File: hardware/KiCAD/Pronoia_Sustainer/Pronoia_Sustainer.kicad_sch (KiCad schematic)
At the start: 0 parts

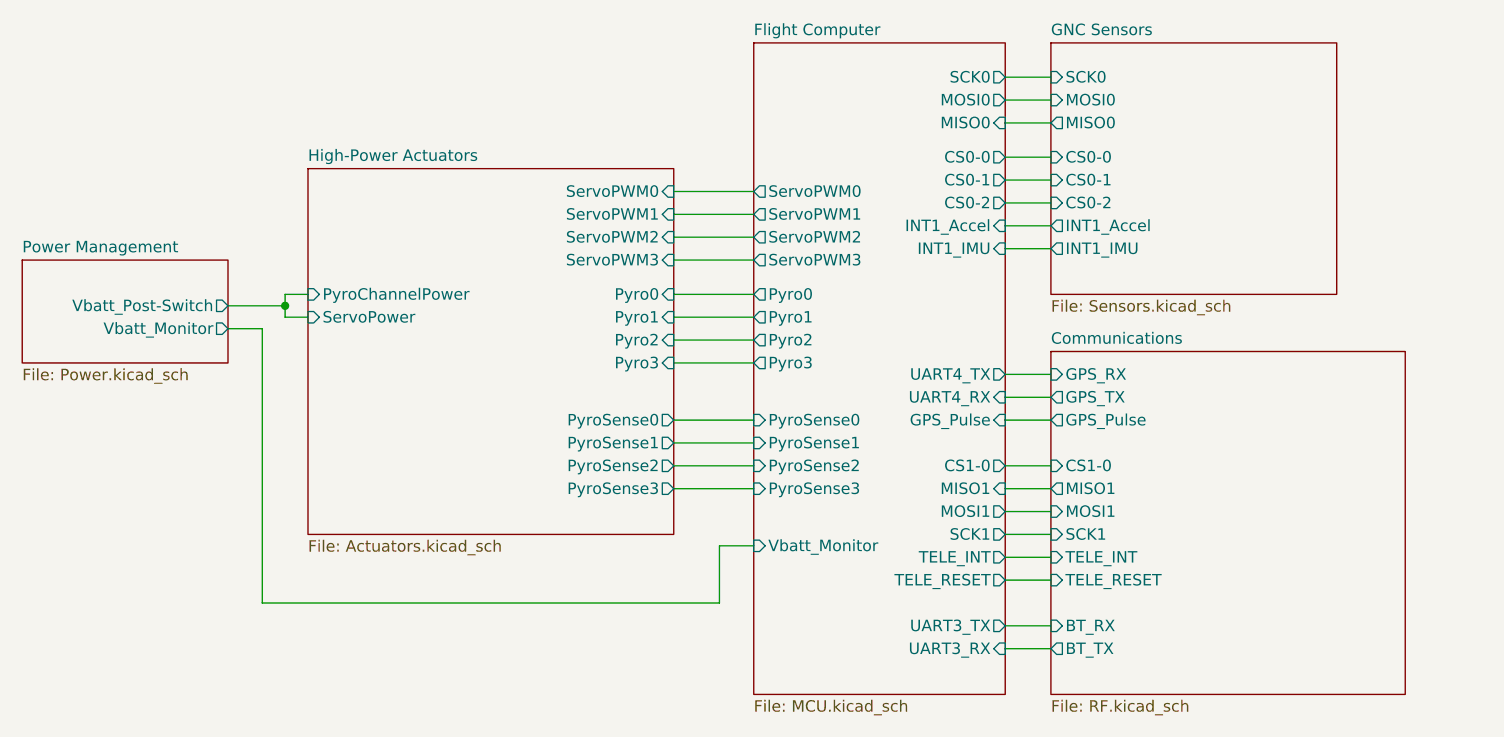
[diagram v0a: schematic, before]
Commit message: Finalized v2.0 of Pronoia Schematic
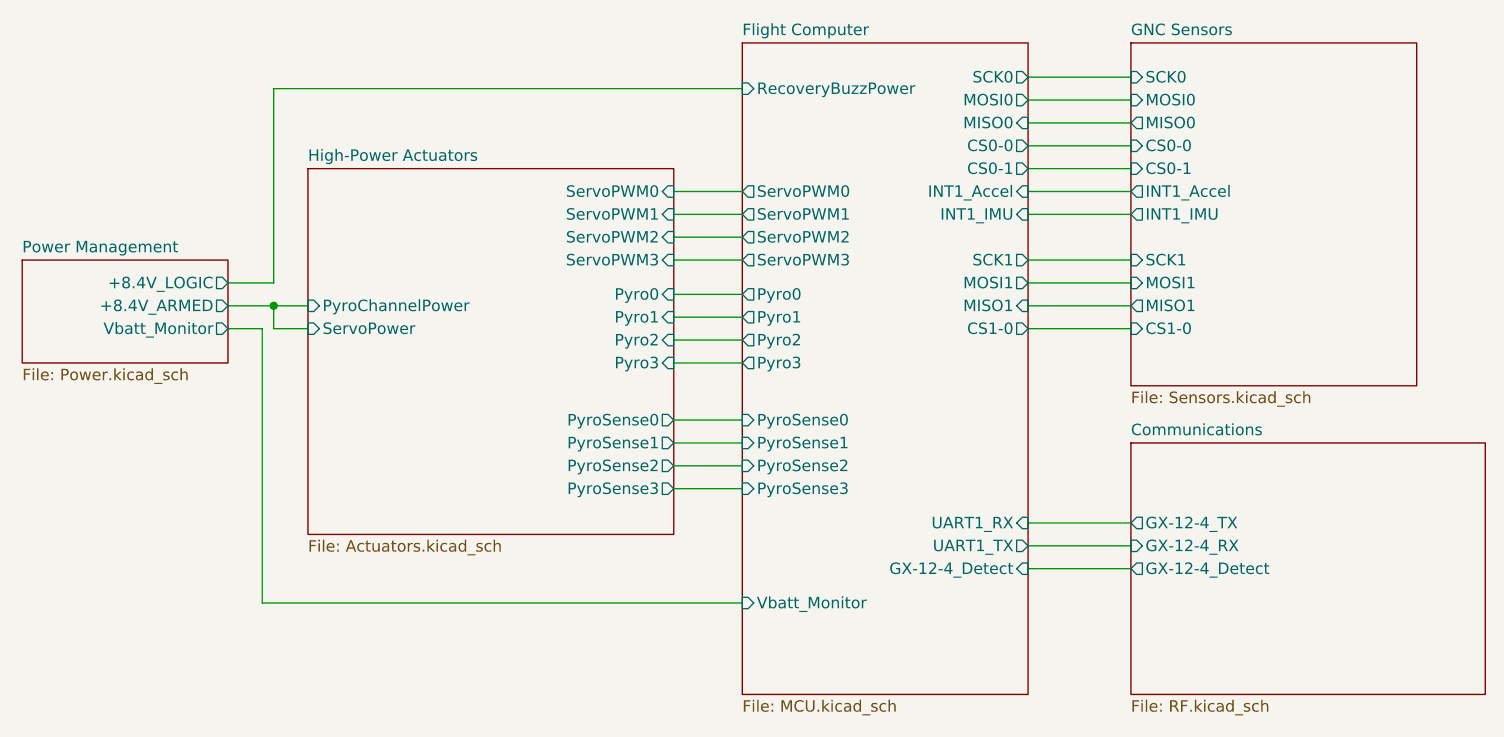
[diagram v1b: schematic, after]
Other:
- sheet Communications ports: added GX-12-4_Detect, GX-12-4_RX, GX-12-4_TX; removed BT_RX, BT_TX, CS1-0, GPS_Pulse, GPS_RX, GPS_TX, MISO1, MOSI1, SCK1, TELE_INT, TELE_RESET
- sheet Flight Computer ports: added GX-12-4_Detect, RecoveryBuzzPower, UART1_RX, UART1_TX; removed CS0-2, GPS_Pulse, TELE_INT, TELE_RESET, UART3_RX, UART3_TX, UART4_RX, UART4_TX
- sheet GNC Sensors ports: added CS1-0, MISO1, MOSI1, SCK1; removed CS0-2
- sheet Power Management ports: added +8.4V_ARMED, +8.4V_LOGIC; removed Vbatt_Post-Switch
